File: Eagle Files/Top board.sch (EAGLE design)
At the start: 3 parts, among them J1 MINI-USB-5P-3400030P1, U1 CN3065-1320040P1

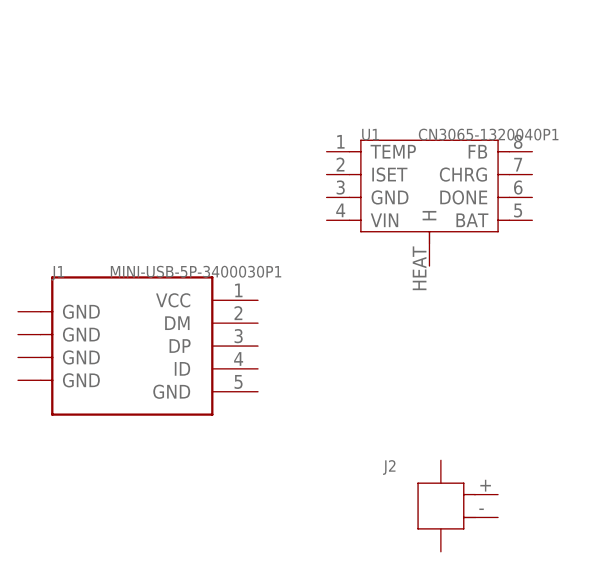
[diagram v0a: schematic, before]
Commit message: Tweak board
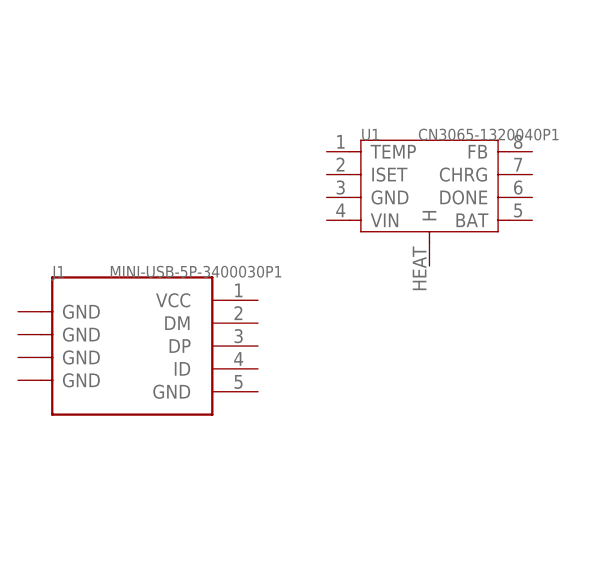
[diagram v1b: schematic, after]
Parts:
- removed J2: (no value), Connector:JST-2P-SMD'2.0'
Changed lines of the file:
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@@
 <setting verticaltext="up"/>
 </settings>
-<grid distance="0.1" unitdist="inch" unit="inch" style="lines" multiple="1" display="no" altdistance="0.01" altunitdist="inch" altunit="inch"/>
+<grid distance="5" unitdist="mil" unit="mil" style="lines" multiple="1" display="no" altdistance="1" altunitdist="mil" altunit="mil"/>
 <layers>
 <layer number="1" name="Top" color="4" fill="1" visible="no" active="no"/>
@@
 <part name="U1" library="IC" deviceset="CN3065" device="-1320040P1"/>
 <part name="J1" library="Connector" deviceset="MINI-USB-5P" device="-3400030P1"/>
-<part name="J2" library="Connector" deviceset="JST-2P-SMD" device="'2.0'"/>
 </parts>
 <sheets>
@@
 <instance part="U1" gate="U" x="73.66" y="58.42"/>
 <instance part="J1" gate="USB" x="40.64" y="40.64"/>
-<instance part="J2" gate="G$1" x="78.74" y="22.86"/>
 </instances>
 <busses>

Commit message: Tweaks
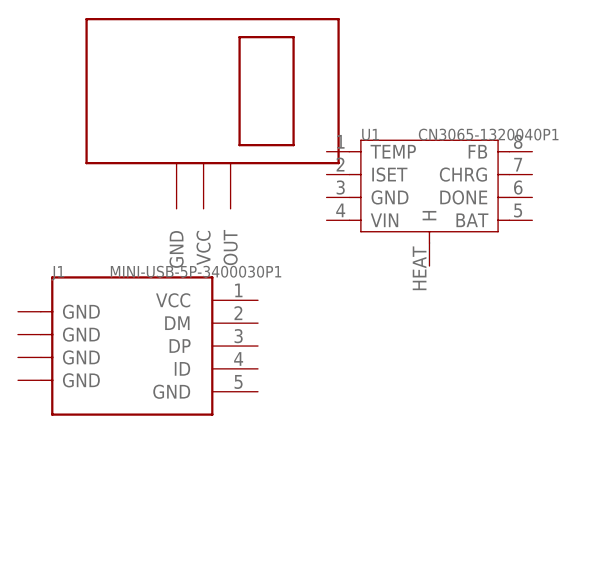
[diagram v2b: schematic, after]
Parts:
- added RD2007: RD2007, radiationbean:RD2007
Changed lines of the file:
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@@
 <setting verticaltext="up"/>
 </settings>
-<grid distance="5" unitdist="mil" unit="mil" style="lines" multiple="1" display="no" altdistance="1" altunitdist="mil" altunit="mil"/>
+<grid distance="0.1" unitdist="inch" unit="inch" style="lines" multiple="1" display="no" altdistance="0.01" altunitdist="inch" altunit="inch"/>
 <layers>
 <layer number="1" name="Top" color="4" fill="1" visible="no" active="no"/>
@@
 <part name="U1" library="IC" deviceset="CN3065" device="-1320040P1"/>
 <part name="J1" library="Connector" deviceset="MINI-USB-5P" device="-3400030P1"/>
+<part name="RD2007" library="radiationbean" deviceset="RD2007" device=""/>
 </parts>
 <sheets>
@@
 <instance part="U1" gate="U" x="73.66" y="58.42"/>
 <instance part="J1" gate="USB" x="40.64" y="40.64"/>
+<instance part="RD2007" gate="G$1" x="35.56" y="60.96"/>
 </instances>
 <busses>
@@
 </schematic>
 </drawing>
+<compatibility>
+<note version="6.3" minversion="6.2.2" severity="warning">
+Since Version 6.2.2 text objects can contain more than one line,
+which will not be processed correctly with this version.
+</note>
+</compatibility>
 </eagle>
